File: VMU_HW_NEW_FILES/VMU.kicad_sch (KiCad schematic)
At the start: 13 parts, among them J1 Conn_01x04_Pin, J10 Conn_01x03_Pin, J11 Conn_01x03_Pin, J12 Conn_01x03_Pin, J13 Conn_01x03_Pin, J14 Conn_01x03_Pin, J2 Conn_01x03_Pin, J3 Conn_01x03_Pin, J4 Conn_01x03_Pin, J5 Conn_01x03_Pin, J7 Conn_01x03_Pin, J8 Conn_01x03_Pin, J9 Conn_01x03_Pin

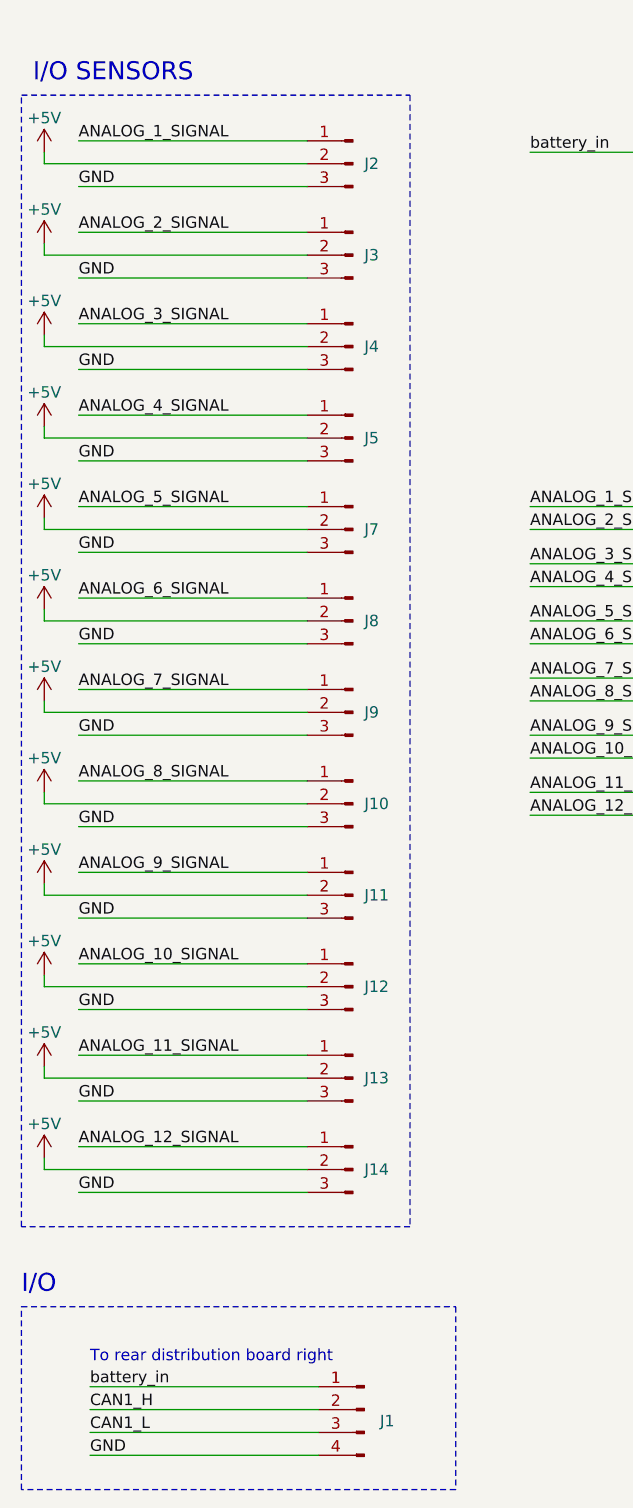
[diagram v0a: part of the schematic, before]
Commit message: VMU small update
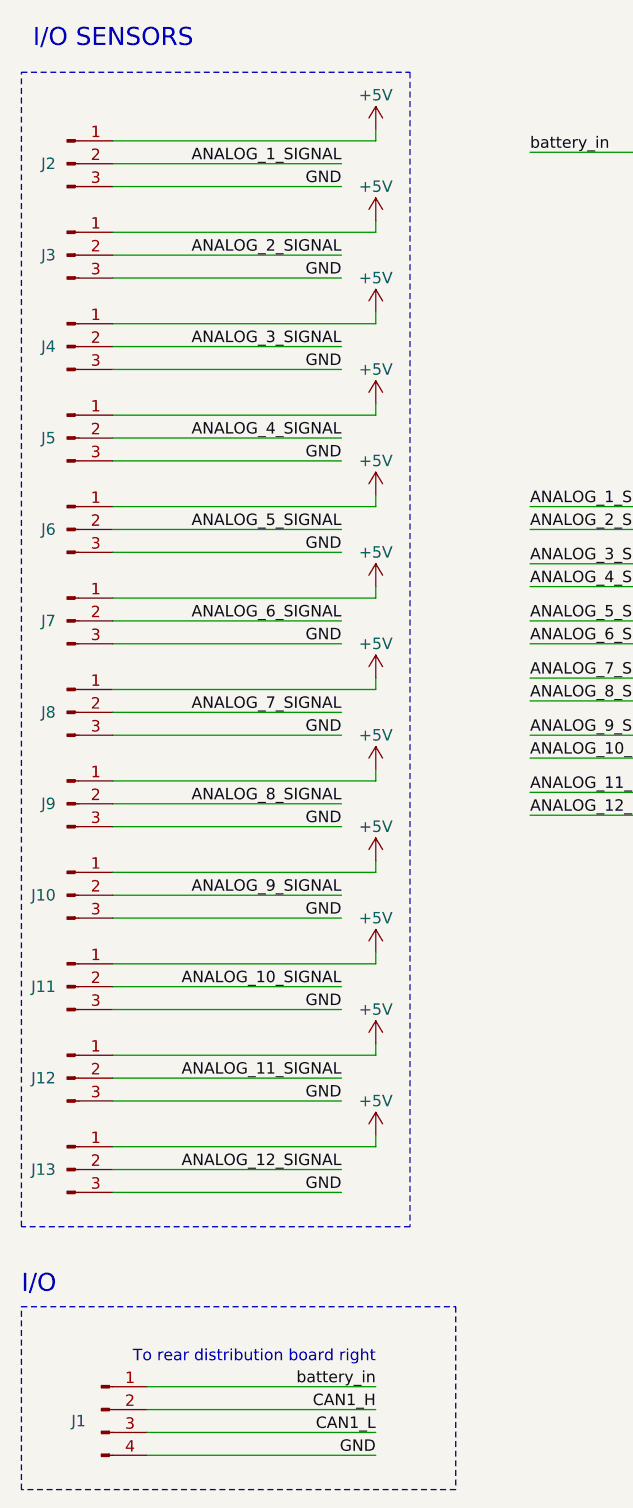
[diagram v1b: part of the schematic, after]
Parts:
- removed J14: Conn_01x03_Pin, symbol Connector:Conn_01x03_Pin
- added J6: Conn_01x03_Pin, symbol Connector:Conn_01x03_Pin
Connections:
- net +5V: now also J10.1 (Pin_1), J11.1 (Pin_1), J12.1 (Pin_1), J13.1 (Pin_1), J2.1 (Pin_1), J3.1 (Pin_1), J4.1 (Pin_1), J5.1 (Pin_1), J7.1 (Pin_1), J8.1 (Pin_1), J9.1 (Pin_1), J6.1 (Pin_1); no longer J10.2 (Pin_2), J11.2 (Pin_2), J12.2 (Pin_2), J13.2 (Pin_2), J2.2 (Pin_2), J3.2 (Pin_2), J4.2 (Pin_2), J5.2 (Pin_2), J7.2 (Pin_2), J8.2 (Pin_2), J9.2 (Pin_2)
- net ANALOG_10_SIGNAL: now also J11.2 (Pin_2); no longer J12.1 (Pin_1)
- net ANALOG_11_SIGNAL: now also J12.2 (Pin_2); no longer J13.1 (Pin_1)
- net ANALOG_12_SIGNAL: now also J13.2 (Pin_2)
- net ANALOG_1_SIGNAL: now also J2.2 (Pin_2); no longer J2.1 (Pin_1)
- net ANALOG_2_SIGNAL: now also J3.2 (Pin_2); no longer J3.1 (Pin_1)
- net ANALOG_3_SIGNAL: now also J4.2 (Pin_2); no longer J4.1 (Pin_1)
- net ANALOG_4_SIGNAL: now also J5.2 (Pin_2); no longer J5.1 (Pin_1)
- net ANALOG_5_SIGNAL: now also J6.2 (Pin_2); no longer J7.1 (Pin_1)
- net ANALOG_6_SIGNAL: now also J7.2 (Pin_2); no longer J8.1 (Pin_1)
- net ANALOG_7_SIGNAL: now also J8.2 (Pin_2); no longer J9.1 (Pin_1)
- net ANALOG_8_SIGNAL: now also J9.2 (Pin_2); no longer J10.1 (Pin_1)
- net ANALOG_9_SIGNAL: now also J10.2 (Pin_2); no longer J11.1 (Pin_1)
- net GND: now also J6.3 (Pin_3)
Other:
- moved on the sheet: J1, J2
